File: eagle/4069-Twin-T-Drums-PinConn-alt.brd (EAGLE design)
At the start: 48.3 x 33 mm, 27 parts, among them IC2 4069N

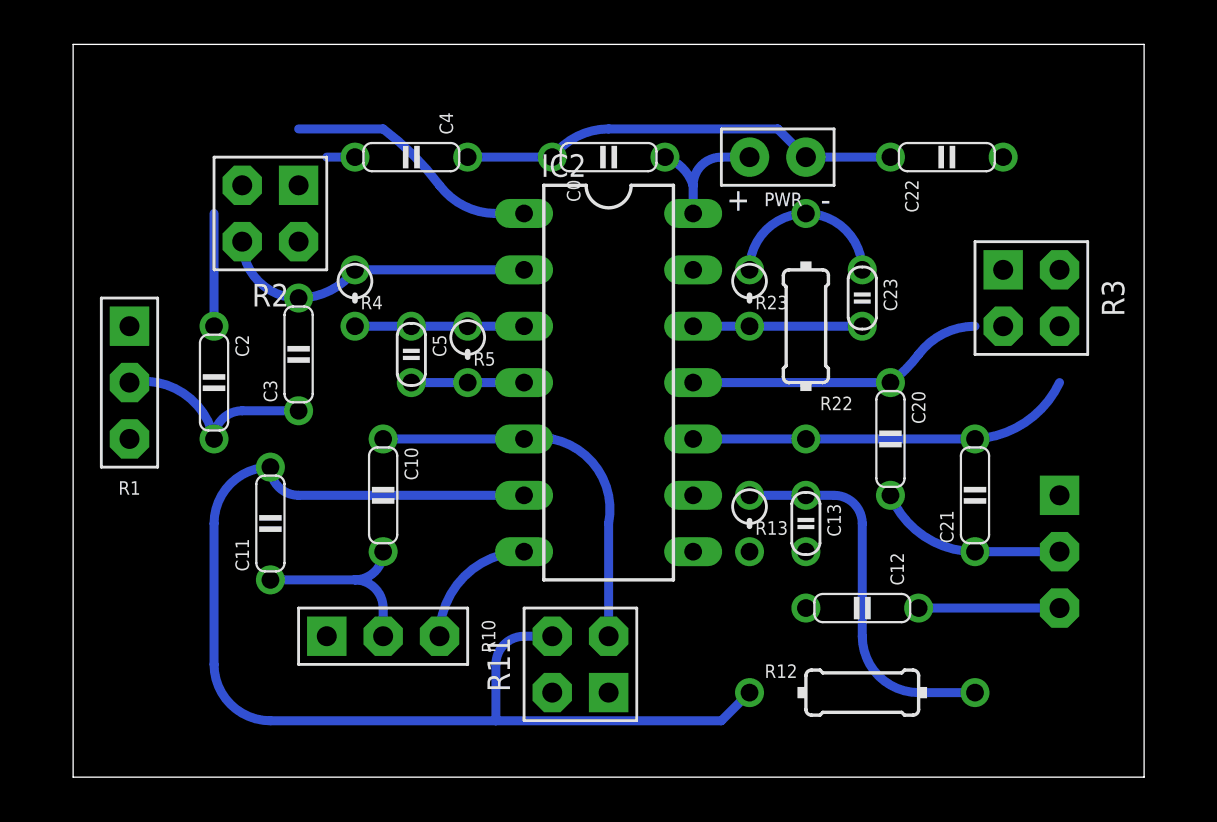
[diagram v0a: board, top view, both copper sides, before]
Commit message: ...
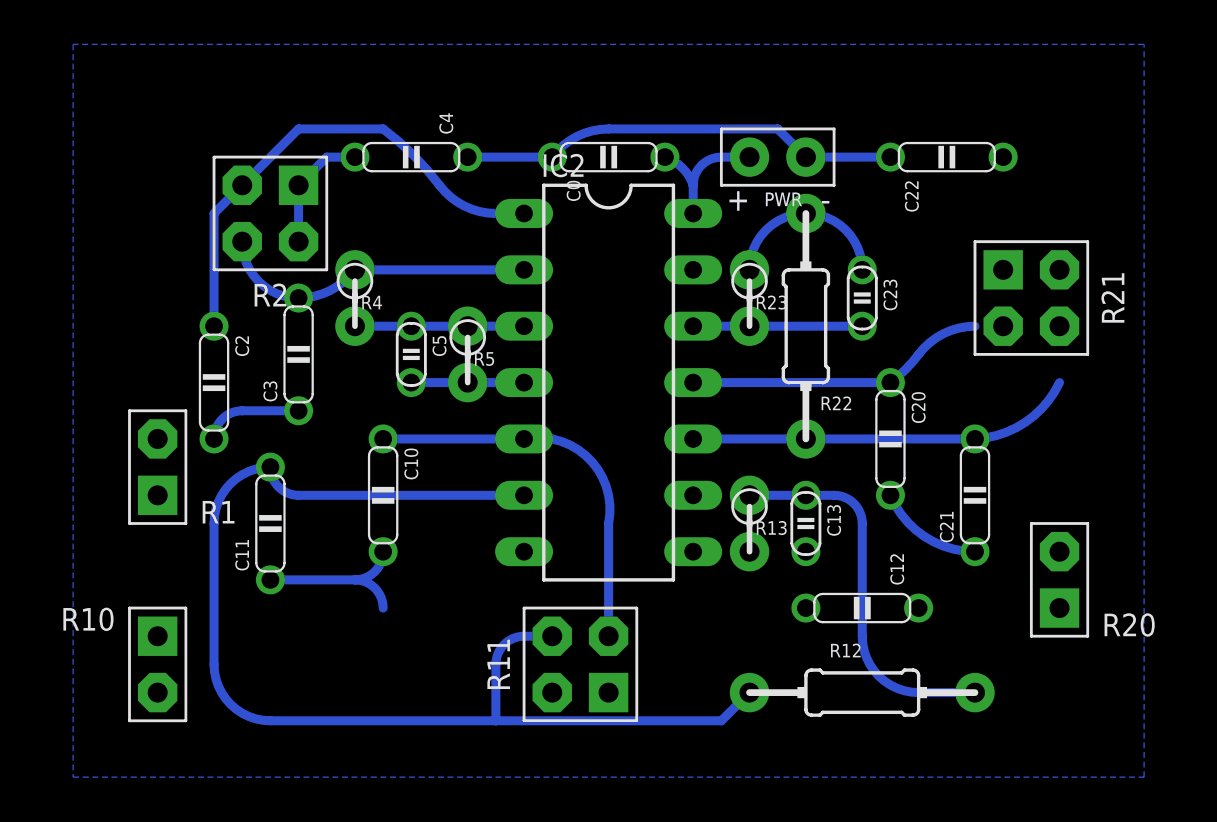
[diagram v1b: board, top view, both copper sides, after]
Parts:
- R1, R10, R20: value 100kΩ -> VAR-V; device r:CONN-3P -> r:CONN-2P
- moved R10 10.2 mm to (11.4, 15.2), turned to 180 degrees
- moved R1 4.02 mm to (11.4, 24.1), turned to 0 degrees
- moved R20 1.27 mm to (52.1, 19.1), flipped to the top, turned to 0 degrees
- renumbered R3 to R21
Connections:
- net GND: now also R1.1, R10.1, R20.1; no longer R1.3, R10.3, R20.3
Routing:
- net GND: track 31.6 -> 19.9 mm
- net I1: track 16.6 -> 22.0 mm
- net TR1: track 8.92 -> 4.34 mm
- net DR1: track 1.27 -> 5.61 mm
- net TR3: track 8.39 -> 4.58 mm
- net TR2: track 8.67 -> 7.40 mm
- added copper zone on layer 16, net N$3
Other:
- board outline removed
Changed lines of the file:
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@@
 <layer number="45" name="Holes" color="7" fill="1" visible="no" active="yes"/>
 <layer number="46" name="Milling" color="3" fill="1" visible="no" active="yes"/>
-<layer number="47" name="Measures" color="7" fill="1" visible="no" active="yes"/>
+<layer number="47" name="Measures" color="7" fill="1" visible="yes" active="yes"/>
 <layer number="48" name="Document" color="7" fill="1" visible="yes" active="yes"/>
 <layer number="49" name="Reference" color="7" fill="1" visible="yes" active="yes"/>
@@
 <board>
 <plain>
-<wire x1="7.62" y1="10.16" x2="55.88" y2="10.16" width="0" layer="20"/>
-<wire x1="55.88" y1="10.16" x2="55.88" y2="43.18" width="0" layer="20"/>
-<wire x1="55.88" y1="43.18" x2="7.62" y2="43.18" width="0" layer="20"/>
-<wire x1="7.62" y1="43.18" x2="7.62" y2="10.16" width="0" layer="20"/>
+<wire x1="7.62" y1="10.16" x2="55.88" y2="10.16" width="0" layer="47"/>
+<wire x1="55.88" y1="10.16" x2="55.88" y2="43.18" width="0" layer="47"/>
+<wire x1="55.88" y1="43.18" x2="7.62" y2="43.18" width="0" layer="47"/>
+<wire x1="7.62" y1="43.18" x2="7.62" y2="10.16" width="0" layer="47"/>
 </plain>
 <attributes>
@@
 <element name="C0" library="c" package="C050-020X044/V" value="100nF" x="31.75" y="38.1" rot="R90"/>
 <element name="IC2" library="ic" package="DIL14" value="4069N" x="31.75" y="27.94"/>
-<element name="R1" library="r" package="CONN-3P" value="100kΩ" x="10.16" y="27.94" rot="R180"/>
-<element name="R10" library="r" package="CONN-3P" value="100kΩ" x="21.59" y="16.51" rot="R270"/>
 <element name="R12" library="r" package="0204/10" value="" x="43.18" y="13.97"/>
 <element name="R13" library="r" package="0202/2V" value="" x="38.1" y="21.59" rot="R180"/>
-<element name="R20" library="r" package="CONN-3P" value="100kΩ" x="52.07" y="20.32" rot="MR180"/>
 <element name="R22" library="r" package="0204/10-V" value="" x="40.64" y="30.48" rot="R180"/>
 <element name="R23" library="r" package="0202/2V" value="" x="38.1" y="31.75" rot="R180"/>
@@
 <element name="R11" library="r" package="CONN-2X2" value="VAR-STEREO-H" x="31.75" y="13.97" rot="R90"/>
 <element name="R2" library="r" package="CONN-2X2" value="VAR-STEREO-H" x="17.78" y="36.83" rot="R180"/>
-<element name="R3" library="r" package="CONN-2X2" value="VAR-STEREO-H" x="49.53" y="33.02" rot="R270"/>
+<element name="R21" library="r" package="CONN-2X2" value="VAR-STEREO-H" x="49.53" y="33.02" rot="R270"/>
+<element name="R1" library="r" package="CONN-2P" value="VAR-V" x="11.43" y="24.13"/>
+<element name="R10" library="r" package="CONN-2P" value="VAR-V" x="11.43" y="15.24" rot="R180"/>
+<element name="R20" library="r" package="CONN-2P" value="VAR-V" x="52.07" y="19.05"/>
 </elements>
 <signals>
@@
 <wire x1="13.97" y1="35.56" x2="13.97" y2="30.48" width="0.4064" layer="16"/>
 <contactref element="R2" pad="2"/>
-<wire x1="15.24" y1="36.83" x2="17.78" y2="39.37" width="0" layer="19" extent="16-16"/>
-<wire x1="13.97" y1="35.56" x2="15.24" y2="36.83" width="0" layer="19" extent="16-16"/>
+<wire x1="15.24" y1="36.83" x2="17.78" y2="39.37" width="0.4064" layer="16"/>
+<wire x1="15.24" y1="36.83" x2="13.97" y2="35.56" width="0.4064" layer="16"/>
 </signal>
 <signal name="GND">
 <contactref element="C4" pad="1"/>
-<contactref element="R1" pad="3"/>
 <contactref element="C12" pad="1"/>
-<contactref element="R10" pad="3"/>
 <contactref element="C22" pad="1"/>
-<contactref element="R20" pad="3"/>
 <contactref element="IC2" pad="7"/>
 <contactref element="C0" pad="1"/>
@@
 <wire x1="31.75" y1="39.37" x2="29.21" y2="38.1" width="0.4064" layer="16" curve="53.130102"/>
 <wire x1="29.21" y1="38.1" x2="25.4" y2="38.1" width="0.4064" layer="16"/>
-<wire x1="45.72" y1="17.78" x2="52.07" y2="17.78" width="0.4064" layer="16"/>
-<wire x1="24.13" y1="16.51" x2="27.94" y2="20.32" width="0.4064" layer="16" curve="-90"/>
-<wire x1="27.94" y1="20.32" x2="29.21" y2="38.1" width="0" layer="19" extent="1-1"/>
-<wire x1="10.16" y1="25.4" x2="24.13" y2="16.51" width="0" layer="19" extent="1-1"/>
-<wire x1="45.72" y1="17.78" x2="27.94" y2="20.32" width="0" layer="19" extent="1-1"/>
+<contactref element="R10" pad="1"/>
+<contactref element="R20" pad="1"/>
+<contactref element="R1" pad="1"/>
+<wire x1="45.72" y1="17.78" x2="52.07" y2="17.78" width="0" layer="19" extent="1-1"/>
+<wire x1="27.94" y1="20.32" x2="45.72" y2="17.78" width="0" layer="19" extent="1-1"/>
+<wire x1="11.43" y1="22.86" x2="27.94" y2="20.32" width="0" layer="19" extent="1-1"/>
+<wire x1="11.43" y1="16.51" x2="11.43" y2="22.86" width="0" layer="19" extent="1-1"/>
+<wire x1="29.21" y1="38.1" x2="27.94" y2="20.32" width="0" layer="19" extent="1-1"/>
 </signal>
 <signal name="I2">
@@
 <contactref element="R2" pad="1"/>
 <contactref element="R2" pad="3"/>
-<wire x1="17.78" y1="36.83" x2="19.05" y2="38.1" width="0" layer="19" extent="16-16"/>
-<wire x1="17.78" y1="34.29" x2="17.78" y2="36.83" width="0" layer="19" extent="1-1"/>
+<wire x1="17.78" y1="34.29" x2="17.78" y2="36.83" width="0.4064" layer="16"/>
+<wire x1="19.05" y1="38.1" x2="17.78" y2="36.83" width="0.4064" layer="16"/>
 </signal>
 <signal name="TR1">
-<contactref element="R1" pad="2"/>
 <contactref element="C2" pad="2"/>
 <contactref element="C3" pad="1"/>
-<wire x1="13.97" y1="25.4" x2="10.16" y2="27.94" width="0.4064" layer="16" curve="90"/>
 <wire x1="13.97" y1="25.4" x2="15.24" y2="26.67" width="0.4064" layer="16" curve="-90"/>
 <wire x1="15.24" y1="26.67" x2="17.78" y2="26.67" width="0.4064" layer="16"/>
+<contactref element="R1" pad="2"/>
+<wire x1="11.43" y1="25.4" x2="13.97" y2="25.4" width="0" layer="19" extent="1-1"/>
 </signal>
 <signal name="O3">
@@
 </signal>
 <signal name="TR2">
-<contactref element="R10" pad="2"/>
 <contactref element="C10" pad="2"/>
 <contactref element="C11" pad="1"/>
 <wire x1="16.51" y1="19.05" x2="20.32" y2="19.05" width="0.4064" layer="16"/>
 <wire x1="20.32" y1="19.05" x2="21.59" y2="20.32" width="0.4064" layer="16" curve="90"/>
-<wire x1="21.59" y1="16.51" x2="21.59" y2="17.78" width="0.4064" layer="16"/>
 <wire x1="21.59" y1="17.78" x2="20.32" y2="19.05" width="0.4064" layer="16" curve="90"/>
+<contactref element="R10" pad="2"/>
+<wire x1="11.43" y1="13.97" x2="16.51" y2="19.05" width="0" layer="19" extent="1-1"/>
 </signal>
 <signal name="O5">
@@
 <wire x1="40.64" y1="25.4" x2="35.56" y2="25.4" width="0.4064" layer="16"/>
 <wire x1="48.26" y1="25.4" x2="52.07" y2="27.94" width="0.4064" layer="16" curve="61.927575"/>
-<contactref element="R3" pad="4"/>
+<contactref element="R21" pad="4"/>
 <wire x1="52.07" y1="27.94" x2="52.07" y2="30.48" width="0" layer="19" extent="16-16"/>
 </signal>
@@
 <wire x1="45.72" y1="29.21" x2="44.45" y2="27.94" width="0.4064" layer="16" curve="-16.260205"/>
 <wire x1="44.45" y1="27.94" x2="35.56" y2="27.94" width="0.4064" layer="16"/>
-<contactref element="R3" pad="2"/>
+<contactref element="R21" pad="2"/>
 <wire x1="48.26" y1="30.48" x2="49.53" y2="30.48" width="0" layer="19" extent="16-16"/>
 </signal>
@@
 </signal>
 <signal name="TR3">
-<contactref element="R20" pad="2"/>
 <contactref element="C20" pad="2"/>
 <contactref element="C21" pad="1"/>
-<wire x1="52.07" y1="20.32" x2="48.26" y2="20.32" width="0.4064" layer="16"/>
 <wire x1="48.26" y1="20.32" x2="44.45" y2="22.86" width="0.4064" layer="16" curve="-67.380135"/>
+<contactref element="R20" pad="2"/>
+<wire x1="48.26" y1="20.32" x2="52.07" y2="20.32" width="0" layer="19" extent="1-1"/>
 </signal>
 <signal name="VCC">
@@
 <signal name="N$2">
 <contactref element="C22" pad="2"/>
-<contactref element="R3" pad="3"/>
-<contactref element="R3" pad="1"/>
+<contactref element="R21" pad="3"/>
+<contactref element="R21" pad="1"/>
 <wire x1="49.53" y1="33.02" x2="49.53" y2="38.1" width="0" layer="19" extent="1-1"/>
 <wire x1="52.07" y1="33.02" x2="49.53" y2="33.02" width="0" layer="19" extent="1-1"/>
 </signal>
+<signal name="N$3">
+<polygon width="0" layer="16">
+<vertex x="7.62" y="43.18"/>
+<vertex x="7.62" y="10.16"/>
+<vertex x="55.88" y="10.16"/>
+<vertex x="55.88" y="43.18"/>
+</polygon>
+</signal>
 </signals>

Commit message: ...
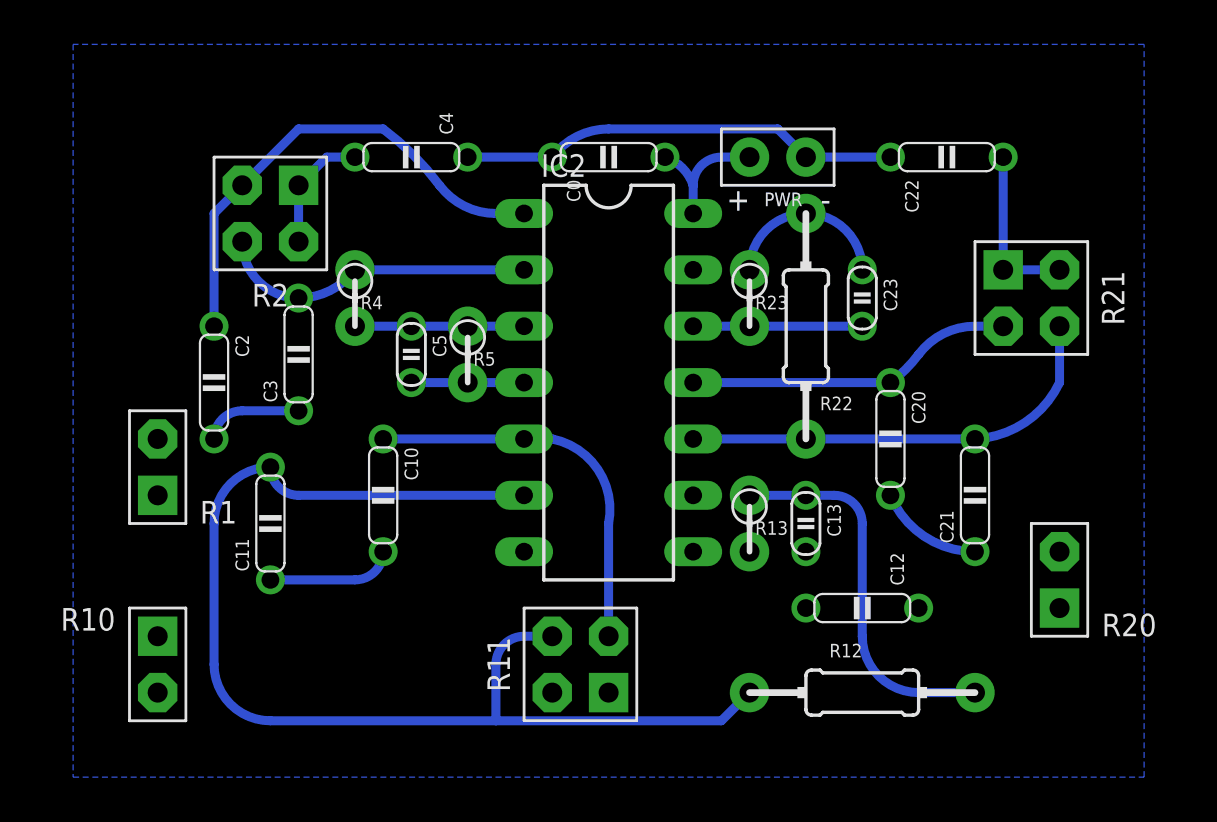
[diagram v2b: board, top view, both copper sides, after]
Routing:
- net N$2: track 0.00 -> 7.62 mm
- net O5: track 17.3 -> 19.8 mm
- net TR2: track 7.40 -> 5.61 mm
- net I5: track 13.5 -> 14.8 mm
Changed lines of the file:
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@@
 <wire x1="16.51" y1="19.05" x2="20.32" y2="19.05" width="0.4064" layer="16"/>
 <wire x1="20.32" y1="19.05" x2="21.59" y2="20.32" width="0.4064" layer="16" curve="90"/>
-<wire x1="21.59" y1="17.78" x2="20.32" y2="19.05" width="0.4064" layer="16" curve="90"/>
 <contactref element="R10" pad="2"/>
 <wire x1="11.43" y1="13.97" x2="16.51" y2="19.05" width="0" layer="19" extent="1-1"/>
@@
 <wire x1="48.26" y1="25.4" x2="52.07" y2="27.94" width="0.4064" layer="16" curve="61.927575"/>
 <contactref element="R21" pad="4"/>
-<wire x1="52.07" y1="27.94" x2="52.07" y2="30.48" width="0" layer="19" extent="16-16"/>
+<wire x1="52.07" y1="27.94" x2="52.07" y2="30.48" width="0.4064" layer="16"/>
 </signal>
 <signal name="I5">
@@
 <wire x1="44.45" y1="27.94" x2="35.56" y2="27.94" width="0.4064" layer="16"/>
 <contactref element="R21" pad="2"/>
-<wire x1="48.26" y1="30.48" x2="49.53" y2="30.48" width="0" layer="19" extent="16-16"/>
+<wire x1="48.26" y1="30.48" x2="49.53" y2="30.48" width="0.4064" layer="16"/>
 </signal>
 <signal name="I6">
@@
 <contactref element="R21" pad="3"/>
 <contactref element="R21" pad="1"/>
-<wire x1="49.53" y1="33.02" x2="49.53" y2="38.1" width="0" layer="19" extent="1-1"/>
-<wire x1="52.07" y1="33.02" x2="49.53" y2="33.02" width="0" layer="19" extent="1-1"/>
+<wire x1="49.53" y1="33.02" x2="52.07" y2="33.02" width="0.4064" layer="16"/>
+<wire x1="49.53" y1="33.02" x2="49.53" y2="38.1" width="0.4064" layer="16"/>
 </signal>
 <signal name="N$3">
